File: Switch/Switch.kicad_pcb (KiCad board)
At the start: 2 copper layers, 22.1 x 128.4 mm, 17 parts, among them SW1 SW_SPDT, SW2 SW_SPDT

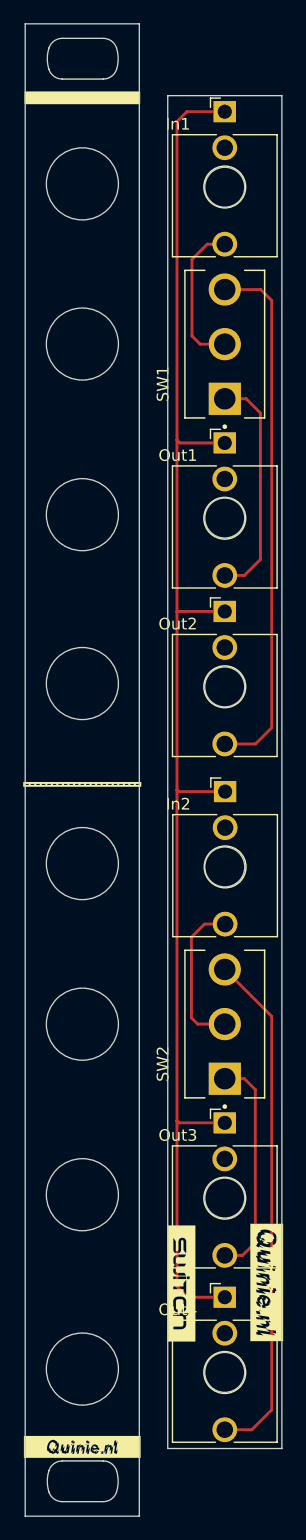
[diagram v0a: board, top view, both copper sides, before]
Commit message: GND
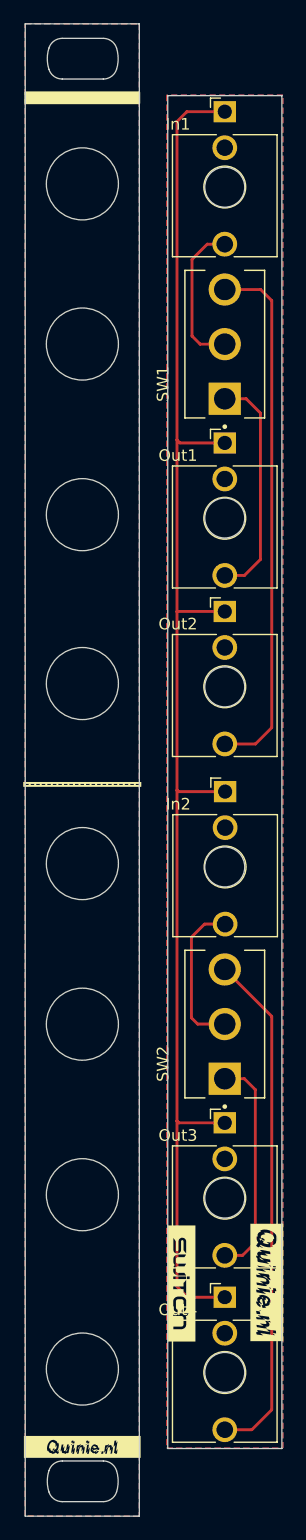
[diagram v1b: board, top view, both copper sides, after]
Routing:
- added copper zone on B.Cu, net (none)
- added copper zone on F.Cu, net (none)
- added copper zone on B.Cu, net GND
- added copper zone on F.Cu, net GND
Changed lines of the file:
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@@
     (attr board_only exclude_from_pos_files exclude_from_bom)
     (fp_text reference "kibuzzard-6564E629" (at 0 4.46148 90) (layer "B.SilkS") hide
-        (effects (font (size 0 0)) (justify mirror))
+        (effects (font (size 0 0) (thickness 0.15)) (justify mirror))
     )
     (fp_text value "G***" (at 0 -4.46148 90) (layer "B.SilkS") hide
-        (effects (font (size 0 0)) (justify mirror))
+        (effects (font (size 0 0) (thickness 0.15)) (justify mirror))
     )
     (fp_poly
@@
   (segment (start 45.29 104.34) (end 45.29 138.19) (width 0.25) (layer "F.Cu") (net 12))
   (segment (start 45.29 138.19) (end 43.58 139.9) (width 0.25) (layer "F.Cu") (net 12))
+  (zone (net 0) (net_name "") (layers "F&B.Cu") (hatch edge 0.5)
+    (priority 1)
+    (connect_pads (clearance 0.5))
+    (min_thickness 0.25) (filled_areas_thickness no)
+    (fill yes (thermal_gap 0.5) (thermal_bridge_width 0.5) (island_removal_mode 1) (island_area_min 10))
+    (polygon
+      (pts
+        (xy 24.075 18.925)
+        (xy 33.9 18.95)
+        (xy 33.9 147.35)
+        (xy 24.075 147.325)
+      )
+    )
+  )
+  (zone (net 1) (net_name "GND") (layers "F&B.Cu") (hatch edge 0.5)
+    (connect_pads (clearance 0.5))
+    (min_thickness 0.25) (filled_areas_thickness no)
+    (fill yes (thermal_gap 0.5) (thermal_bridge_width 0.5))
+    (polygon
+      (pts
+        (xy 46.25 25.075)
+        (xy 36.25 25.075)
+        (xy 36.25 141.475)
+        (xy 46.25 141.475)
+      )
+    )
+  )
 )
